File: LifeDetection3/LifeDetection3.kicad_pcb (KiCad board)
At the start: 2 copper layers, 101.6 x 83.8 mm, 27 parts, among them J1 Power, J12 XT60PW-M, J2 PWM, J3 Analog, J4 PWM, J5 Analog, J6 Communication, J7 Digital, P10 CONN_01X01, P8 CONN_01X01, P9 CONN_01X01, U1 TLP3545

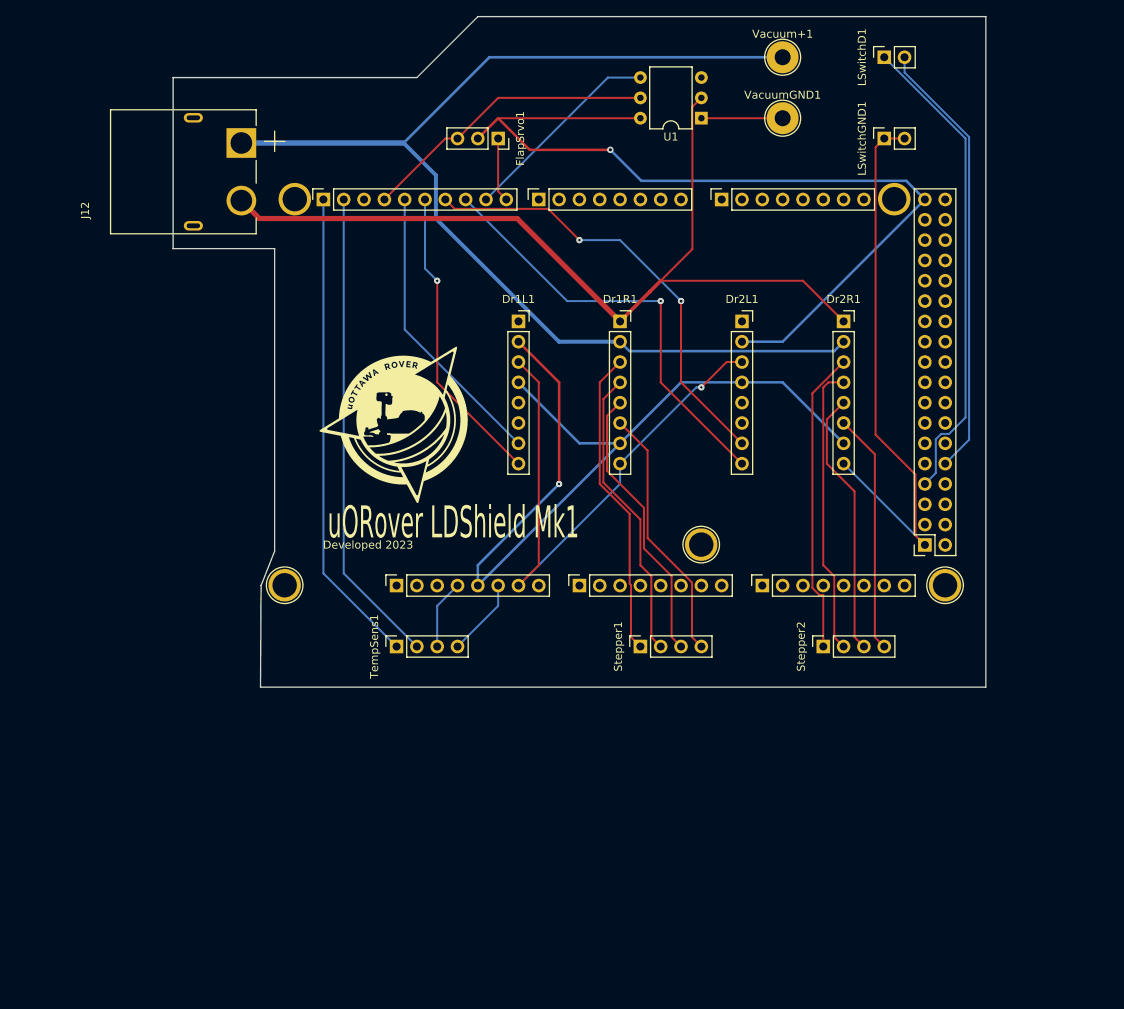
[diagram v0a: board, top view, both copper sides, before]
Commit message: final touches
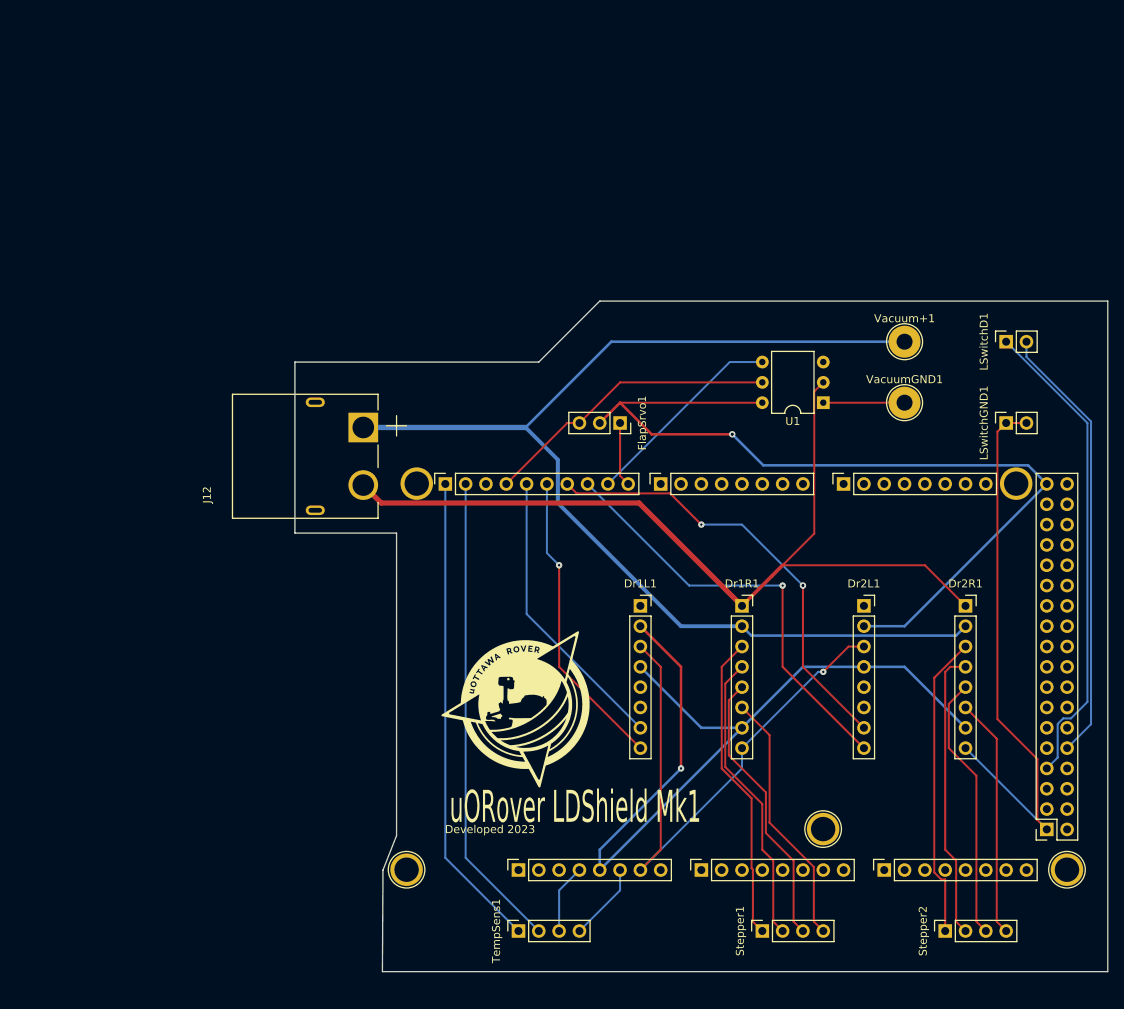
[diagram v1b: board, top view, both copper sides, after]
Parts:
- moved J1 38.7 mm to (143.2, 133.0)
- moved J5 38.7 mm to (188.9, 133.0)
- moved P10 38.7 mm to (211.7, 133.0)
- moved P8 38.7 mm to (129.2, 133.0)
- moved J3 38.7 mm to (166.0, 133.0)
- moved Dr1R1 38.7 mm to (171.1, 100.0)
- moved Dr2L1 38.7 mm to (186.4, 100.0)
- moved Dr2R1 38.7 mm to (199.1, 100.0)
- moved FlapSrvo1 38.7 mm to (155.9, 77.1)
- moved G*** 38.7 mm to (143.2, 112.7)
- moved J2 38.7 mm to (134.0, 84.8)
- moved J4 38.7 mm to (161.0, 84.8)
- moved J7 38.7 mm to (209.2, 127.9)
- moved Vacuum+1 38.7 mm to (191.4, 67.0)
- moved ? 38.7 mm to (130.5, 84.7)
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
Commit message: final touches
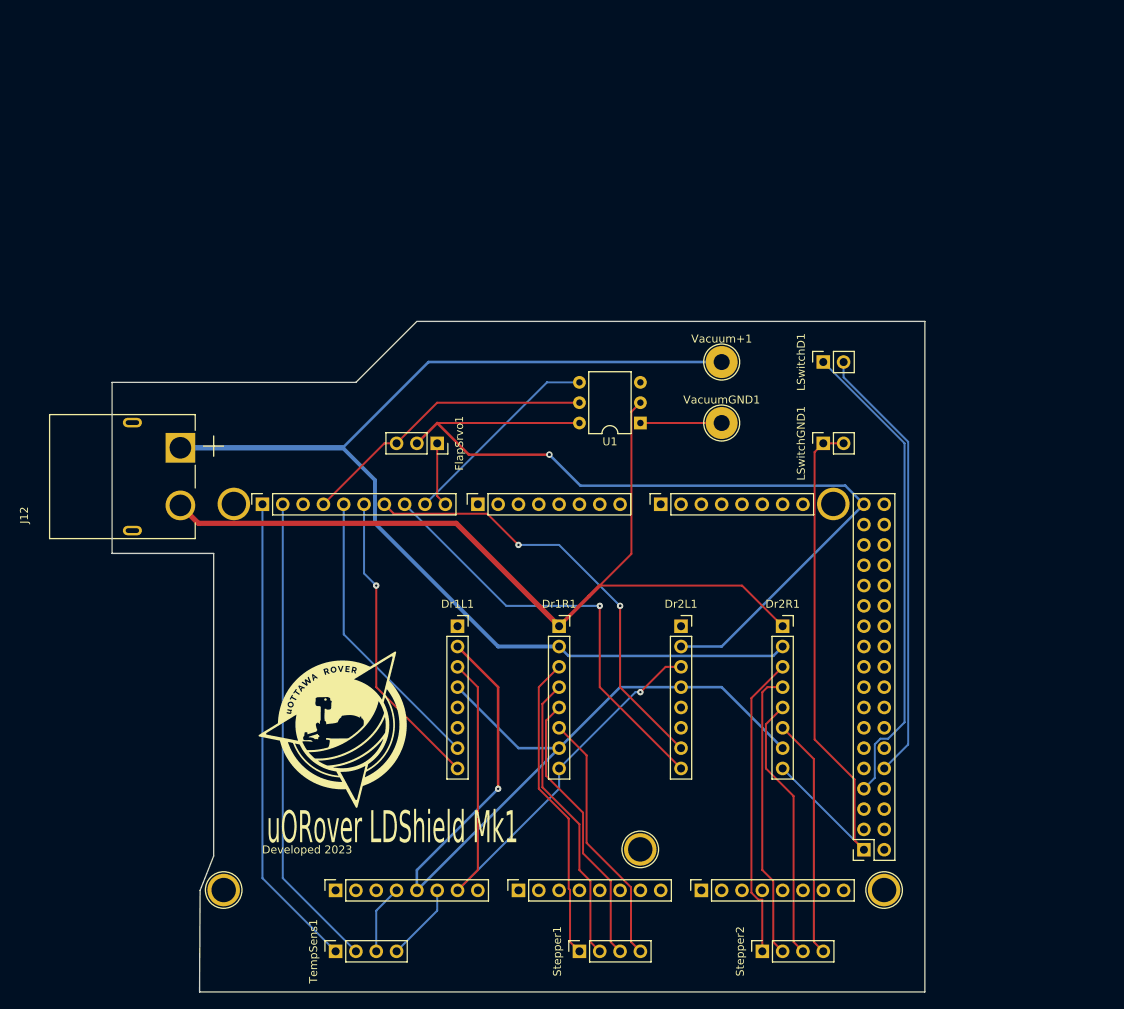
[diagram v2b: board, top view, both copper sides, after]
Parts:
- moved Stepper2 23.0 mm to (173.7, 143.2)
- moved TempSens1 23.0 mm to (120.3, 143.2)
- moved ? 23.0 mm to (107.6, 87.3)
- moved Dr1R1 23.0 mm to (148.3, 102.5)
- moved Dr2L1 23.0 mm to (163.5, 102.5)
- moved Dr2R1 23.0 mm to (176.2, 102.5)
- moved G*** 23.0 mm to (120.3, 115.2)
- moved J1 23.0 mm to (120.3, 135.6)
- moved J4 23.0 mm to (138.1, 87.3)
- moved J5 23.0 mm to (166.0, 135.6)
- moved P10 23.0 mm to (188.9, 135.5)
- moved U1 23.0 mm to (158.4, 77.1)
- moved J12 23.0 mm to (94.9, 83.8)
- moved J2 23.0 mm to (111.2, 87.3)
- moved P8 23.0 mm to (106.3, 135.5)
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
